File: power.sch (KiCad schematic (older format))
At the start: 40 parts, among them J5 Conn_01x02, Q2 AON7405, Q3 Q_NMOS_GSD, U7 MP8759GD, U8 NCP133AMX150TCG

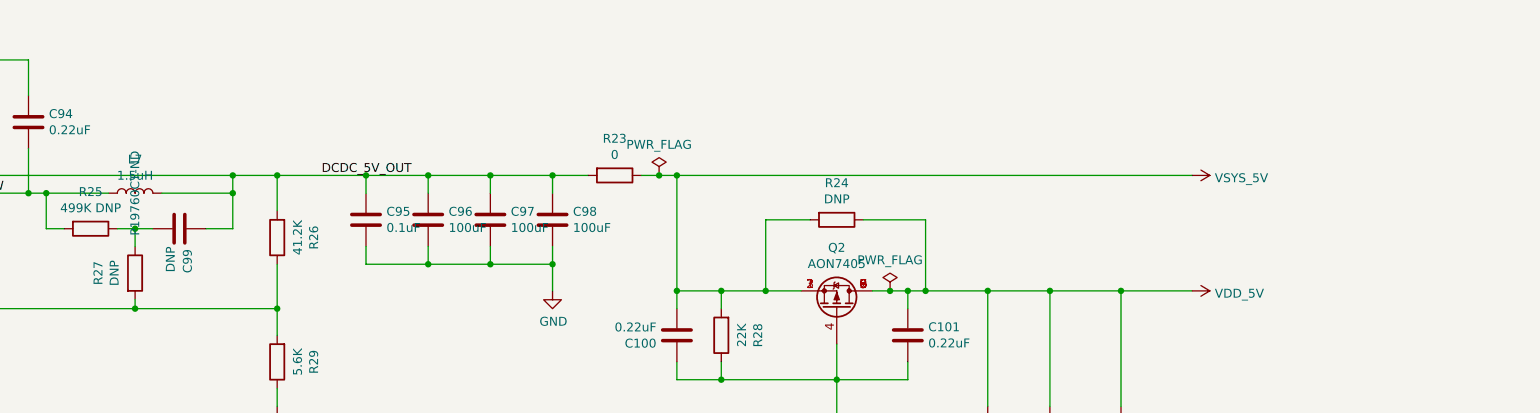
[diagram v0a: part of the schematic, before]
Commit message: wip more new layout
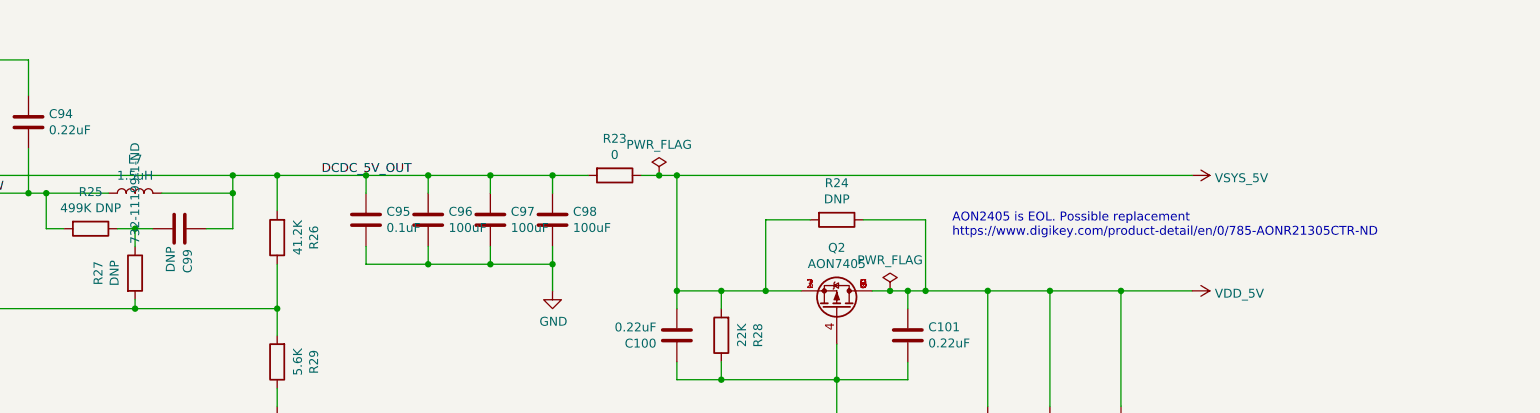
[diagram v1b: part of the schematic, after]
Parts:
- L7: footprint Inductor_SMD:L_6.3x6.3_H3 -> Inductor_SMD:L_Wuerth_MAPI-4020; Mfgr Panasonic -> Würth; Part ETQ-P3M1R5KVP -> 74438357015; Vendorpart P19760CT-ND -> 732-11199-1-ND
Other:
- note added: "AON2405 is EOL. Possible replacement\nhttps://www.digikey.com/product-detail/en/0/785-AONR21305CTR-ND"
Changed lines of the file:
@@
 $Descr USLedger 17000 11000
 encoding utf-8
-Sheet 7 9
+Sheet 7 10
 Title ""
 Date ""
@@
 F 0 "L7" V 8390 2500 50  0000 C CNN
 F 1 "1.5uH" V 8299 2500 50  0000 C CNN
-F 2 "Inductor_SMD:L_6.3x6.3_H3" H 8200 2500 50  0001 C CNN
+F 2 "Inductor_SMD:L_Wuerth_MAPI-4020" H 8200 2500 50  0001 C CNN
 F 3 "~" H 8200 2500 50  0001 C CNN
-F 4 "P19760CT-ND" H 8200 2500 50  0000 C CNN "Vendorpart"
-F 5 "Panasonic" H 8200 2500 50  0001 C CNN "Mfgr"
-F 6 "ETQ-P3M1R5KVP" H 8200 2500 50  0001 C CNN "Part"
+F 4 "732-11199-1-ND" H 8200 2500 50  0000 C CNN "Vendorpart"
+F 5 "Würth" H 8200 2500 50  0001 C CNN "Mfgr"
+F 6 "74438357015" H 8200 2500 50  0001 C CNN "Part"
 	1    8200 2500
 	0    -1   -1   0
@@
 Wire Wire Line
 	3850 2950 4200 2950
+Text Notes 12800 2750 0    50   ~ 0
+AON2405 is EOL. Possible replacement\nhttps://www.digikey.com/product-detail/en/0/785-AONR21305CTR-ND
 $EndSCHEMATC
